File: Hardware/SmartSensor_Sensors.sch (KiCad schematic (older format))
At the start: 13 parts, among them IC1 VEML7700-TT, IC2 SHTC3, Q2 DMG2301L, Q3 DMG2301L, Q4 DMG2301L, U2 CCS811

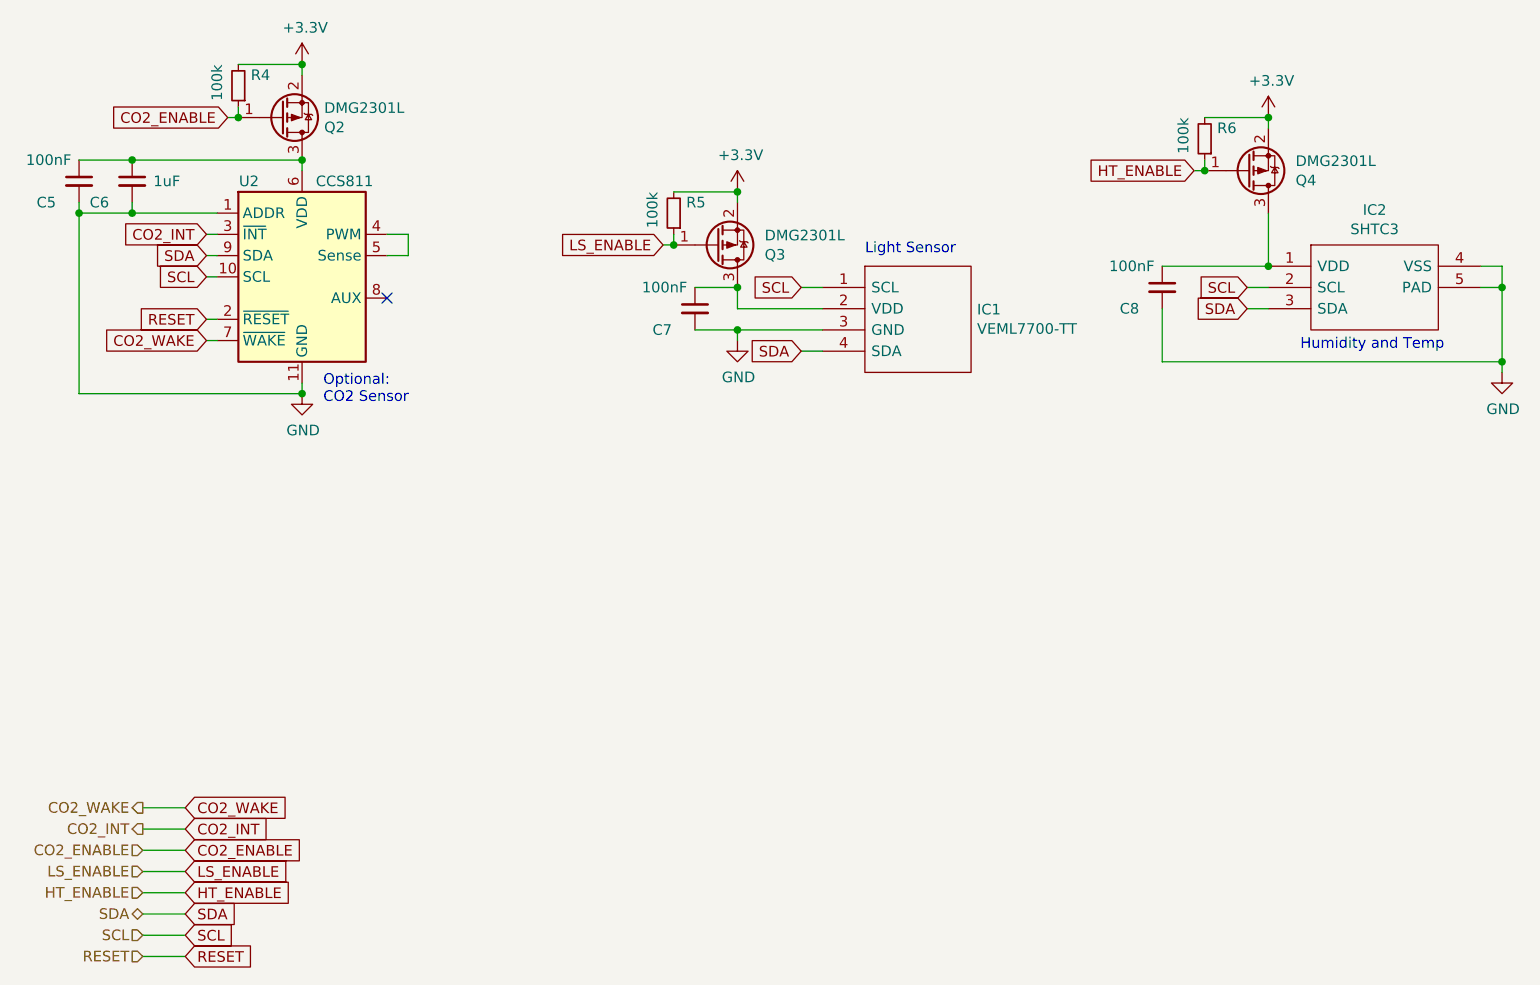
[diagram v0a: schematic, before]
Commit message: Added final version 1.2 to the repository
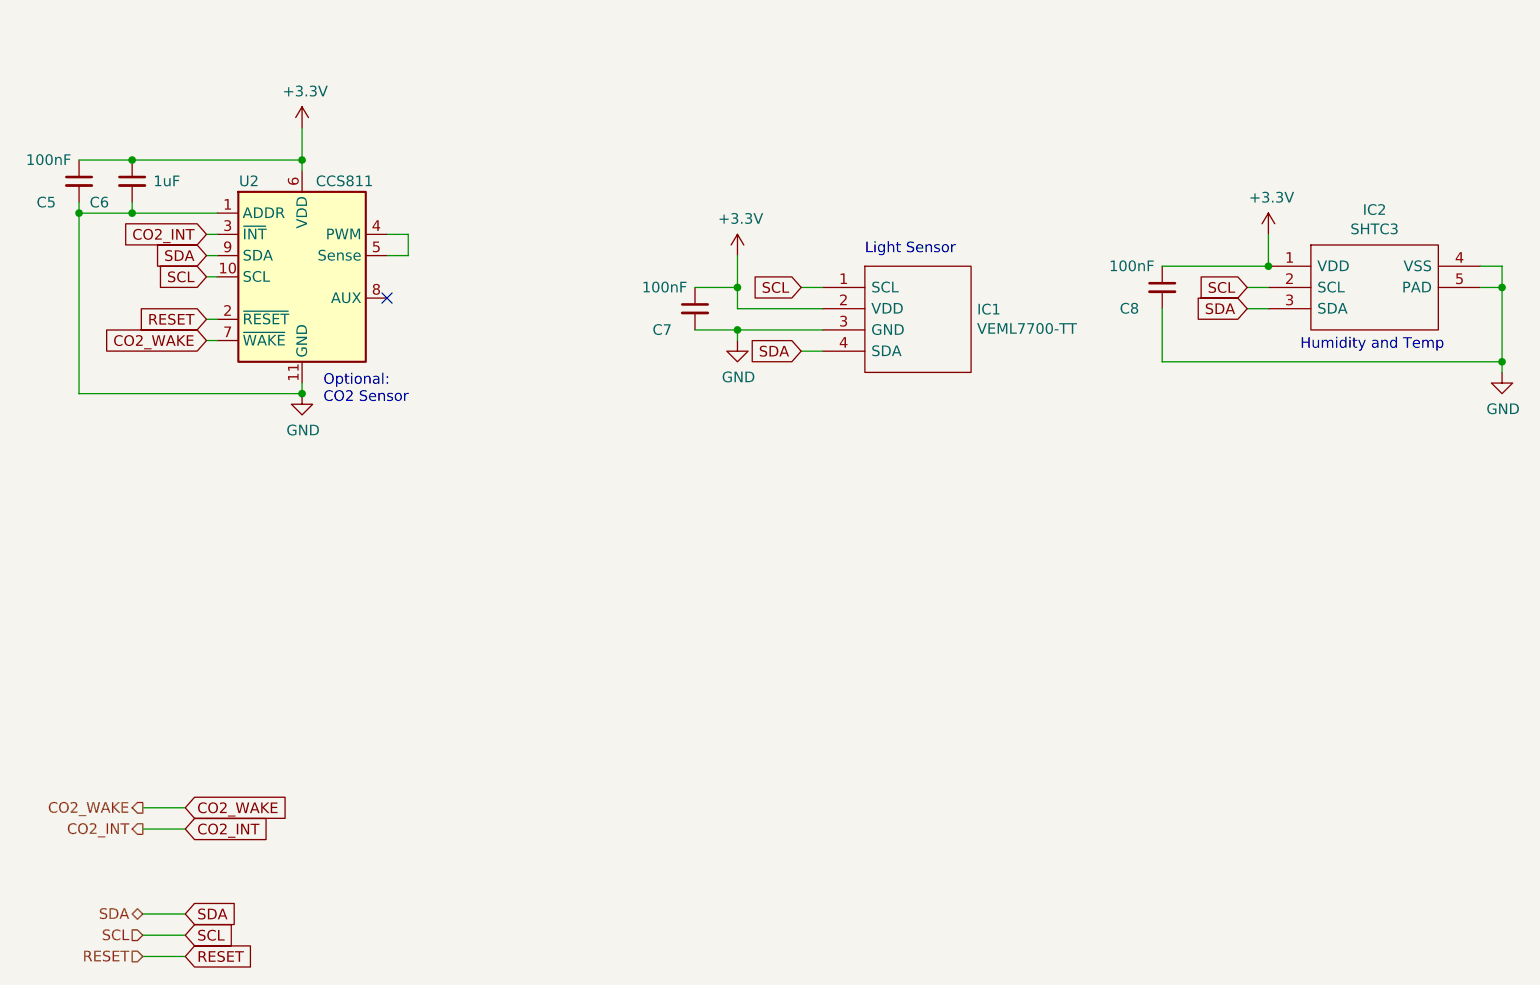
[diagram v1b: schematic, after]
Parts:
- removed Q2, Q3, Q4: DMG2301L, Package_TO_SOT_SMD:SOT-23, symbol Transistor_FET:DMG2301L
- removed R4, R5, R6: 100k, Resistor_SMD:R_0805_2012Metric, symbol Device:R_Small
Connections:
- net +3V3: now also C5.1, C6.1, C7.1, C8.1, IC1.2 (VDD), IC2.1 (VDD), U2.6 (VDD)
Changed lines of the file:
@@
 $Descr A4 11693 8268
 encoding utf-8
-Sheet 3 6
+Sheet 6 6
 Title "SmartSensor"
-Date "2021-03-19"
-Rev "1.1"
+Date "2021-06-14"
+Rev "1.2"
 Comp "Avans Hogeschool"
 Comment1 "Maurice Snoeren"
@@
 $EndComp
 $Comp
-L Transistor_FET:DMG2301L Q?
-U 1 1 5F8743B9
-P 1850 1300
-AR Path="/5F8743B9" Ref="Q?"  Part="1"
-AR Path="/5F86FCBB/5F8743B9" Ref="Q2"  Part="1"
-F 0 "Q2" H 2054 1346 50  0000 L CNN
-F 1 "DMG2301L" H 2054 1255 50  0000 L CNN
-F 2 "Package_TO_SOT_SMD:SOT-23" H 2050 1225 50  0001 L CIN
-F 3 "https://www.diodes.com/assets/Datasheets/DMG2301L.pdf" H 1850 1300 50  0001 L CNN
-	1    1850 1300
-	1    0    0    1
-$EndComp
-$Comp
 L power:+3.3V #PWR?
 U 1 1 5F8743BF
-P 1950 1050
+P 1950 1350
 AR Path="/5F8743BF" Ref="#PWR?"  Part="1"
 AR Path="/5F86FCBB/5F8743BF" Ref="#PWR06"  Part="1"
-F 0 "#PWR06" H 1950 900 50  0001 C CNN
-F 1 "+3.3V" H 1965 1223 50  0000 C CNN
-F 2 "" H 1950 1050 50  0001 C CNN
-F 3 "" H 1950 1050 50  0001 C CNN
-	1    1950 1050
+F 0 "#PWR06" H 1950 1200 50  0001 C CNN
+F 1 "+3.3V" H 1965 1523 50  0000 C CNN
+F 2 "" H 1950 1350 50  0001 C CNN
+F 3 "" H 1950 1350 50  0001 C CNN
+	1    1950 1350
 	1    0    0    -1
 $EndComp
 Text Notes 2050 2650 0    50   ~ 0
 Optional:\nCO2 Sensor
-Wire Wire Line
-	1950 1050 1950 1100
 Wire Wire Line
 	1950 1500 1950 1550
@@
 	1    0    0    -1
 $EndComp
-Text GLabel 1600 1300 0    50   Input ~ 0
-CO2_ENABLE
-Wire Wire Line
-	1600 1300 1650 1300
 Text GLabel 1500 2050 0    50   Input ~ 0
 SCL
@@
 Wire Wire Line
 	1950 1500 1150 1500
-Connection ~ 1950 1500
 Wire Wire Line
 	900  1700 900  1750
@@
 	1150 1750 900  1750
 $Comp
-L Device:R_Small R?
-U 1 1 5F8743F8
-P 1650 1150
-AR Path="/5F8743F8" Ref="R?"  Part="1"
-AR Path="/5F86FCBB/5F8743F8" Ref="R4"  Part="1"
-F 0 "R4" H 1500 1100 50  0000 L CNN
-F 1 "100k" V 1750 1050 50  0000 L CNN
-F 2 "Resistor_SMD:R_0805_2012Metric" H 1650 1150 50  0001 C CNN
-F 3 "~" H 1650 1150 50  0001 C CNN
-	1    1650 1150
-	-1   0    0    1
-$EndComp
-Wire Wire Line
-	1650 1250 1650 1300
-Connection ~ 1650 1300
-$Comp
-L Transistor_FET:DMG2301L Q3
-U 1 1 5F8770D5
-P 3900 1900
-F 0 "Q3" H 4128 1946 50  0000 L CNN
-F 1 "DMG2301L" H 4128 1855 50  0000 L CNN
-F 2 "Package_TO_SOT_SMD:SOT-23" H 4100 1825 50  0001 L CIN
-F 3 "https://www.diodes.com/assets/Datasheets/DMG2301L.pdf" H 3900 1900 50  0001 L CNN
-	1    3900 1900
-	1    0    0    1
-$EndComp
-$Comp
 L power:GND #PWR09
 U 1 1 5F8770DB
@@
 Wire Wire Line
 	3800 2100 4000 2100
-Connection ~ 4000 2100
 Wire Wire Line
 	3800 2300 4000 2300
@@
 L power:+3.3V #PWR08
 U 1 1 5F877100
-P 4000 1650
-F 0 "#PWR08" H 4000 1500 50  0001 C CNN
-F 1 "+3.3V" H 4015 1823 50  0000 C CNN
-F 2 "" H 4000 1650 50  0001 C CNN
-F 3 "" H 4000 1650 50  0001 C CNN
-	1    4000 1650
-	1    0    0    -1
-$EndComp
-Wire Wire Line
-	4000 1650 4000 1700
-Text GLabel 3650 1900 0    50   Input ~ 0
-LS_ENABLE
-Wire Wire Line
-	3650 1900 3700 1900
-$Comp
-L Device:R_Small R5
-U 1 1 5F877109
-P 3700 1750
-F 0 "R5" H 3550 1700 50  0000 L CNN
-F 1 "100k" V 3800 1650 50  0000 L CNN
-F 2 "Resistor_SMD:R_0805_2012Metric" H 3700 1750 50  0001 C CNN
-F 3 "~" H 3700 1750 50  0001 C CNN
-	1    3700 1750
-	-1   0    0    1
-$EndComp
-Wire Wire Line
-	3700 1850 3700 1900
-Connection ~ 3700 1900
-Wire Wire Line
-	3700 1650 4000 1650
-Connection ~ 4000 1650
+P 4000 1950
+F 0 "#PWR08" H 4000 1800 50  0001 C CNN
+F 1 "+3.3V" H 4015 2123 50  0000 C CNN
+F 2 "" H 4000 1950 50  0001 C CNN
+F 3 "" H 4000 1950 50  0001 C CNN
+	1    4000 1950
+	1    0    0    -1
+$EndComp
 $Comp
 L SmartSensor-rescue:SHTC3-SamacSys_Parts IC?
@@
 	1    0    0    -1
 $EndComp
-Connection ~ 1950 1050
-Wire Wire Line
-	1650 1050 1950 1050
-$Comp
-L Transistor_FET:DMG2301L Q4
-U 1 1 5F3CB783
-P 6400 1550
-F 0 "Q4" H 6628 1596 50  0000 L CNN
-F 1 "DMG2301L" H 6628 1505 50  0000 L CNN
-F 2 "Package_TO_SOT_SMD:SOT-23" H 6600 1475 50  0001 L CIN
-F 3 "https://www.diodes.com/assets/Datasheets/DMG2301L.pdf" H 6400 1550 50  0001 L CNN
-	1    6400 1550
-	1    0    0    1
-$EndComp
 $Comp
 L power:+3.3V #PWR010
 U 1 1 5F3CB78D
-P 6500 1300
-F 0 "#PWR010" H 6500 1150 50  0001 C CNN
-F 1 "+3.3V" H 6515 1473 50  0000 C CNN
-F 2 "" H 6500 1300 50  0001 C CNN
-F 3 "" H 6500 1300 50  0001 C CNN
-	1    6500 1300
-	1    0    0    -1
-$EndComp
-Wire Wire Line
-	6500 1300 6500 1350
-Text GLabel 6150 1550 0    50   Input ~ 0
-HT_ENABLE
-Wire Wire Line
-	6150 1550 6200 1550
-$Comp
-L Device:R_Small R6
-U 1 1 5F3CB79A
-P 6200 1400
-F 0 "R6" H 6050 1350 50  0000 L CNN
-F 1 "100k" V 6300 1300 50  0000 L CNN
-F 2 "Resistor_SMD:R_0805_2012Metric" H 6200 1400 50  0001 C CNN
-F 3 "~" H 6200 1400 50  0001 C CNN
-	1    6200 1400
-	-1   0    0    1
-$EndComp
-Wire Wire Line
-	6200 1500 6200 1550
-Connection ~ 6200 1550
-Wire Wire Line
-	6200 1300 6500 1300
-Connection ~ 6500 1300
-Wire Wire Line
-	6500 1750 6500 2000
+P 6500 1850
+F 0 "#PWR010" H 6500 1700 50  0001 C CNN
+F 1 "+3.3V" H 6515 2023 50  0000 C CNN
+F 2 "" H 6500 1850 50  0001 C CNN
+F 3 "" H 6500 1850 50  0001 C CNN
+	1    6500 1850
+	1    0    0    -1
+$EndComp
 $Comp
 L power:GND #PWR011
@@
 Wire Wire Line
 	6000 2000 6500 2000
-Connection ~ 6500 2000
 Wire Wire Line
 	7500 2100 7600 2100
@@
 Text Notes 6650 2400 0    50   ~ 0
 Humidity and Temp
-Text HLabel 1200 4750 0    50   Input ~ 0
-CO2_ENABLE
-Text HLabel 1200 4850 0    50   Input ~ 0
-LS_ENABLE
-Text HLabel 1200 4950 0    50   Input ~ 0
-HT_ENABLE
-Text GLabel 1400 4750 2    50   Input ~ 0
-CO2_ENABLE
-Text GLabel 1400 4850 2    50   Input ~ 0
-LS_ENABLE
-Text GLabel 1400 4950 2    50   Input ~ 0
-HT_ENABLE
 Text HLabel 1200 5050 0    50   BiDi ~ 0
 SDA
@@
 Wire Wire Line
 	1200 4650 1400 4650
-Wire Wire Line
-	1200 4750 1400 4750
-Wire Wire Line
-	1200 4850 1400 4850
-Wire Wire Line
-	1200 4950 1400 4950
 Wire Wire Line
 	1200 5050 1400 5050
@@
 Wire Wire Line
 	4300 2100 4400 2100
+Wire Wire Line
+	1950 1350 1950 1500
+Connection ~ 1950 1500
+Wire Wire Line
+	4000 1950 4000 2100
+Connection ~ 4000 2100
+Wire Wire Line
+	6500 1850 6500 2000
+Connection ~ 6500 2000
 $EndSCHEMATC
